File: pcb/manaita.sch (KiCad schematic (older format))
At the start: 110 parts, among them J1 SCK, J2 RST, J3 MOSI, J4 MISO, J5 VCC, J6 GND, U1 ATmega32U4-AU, Y1 Crystal_GND24_Small

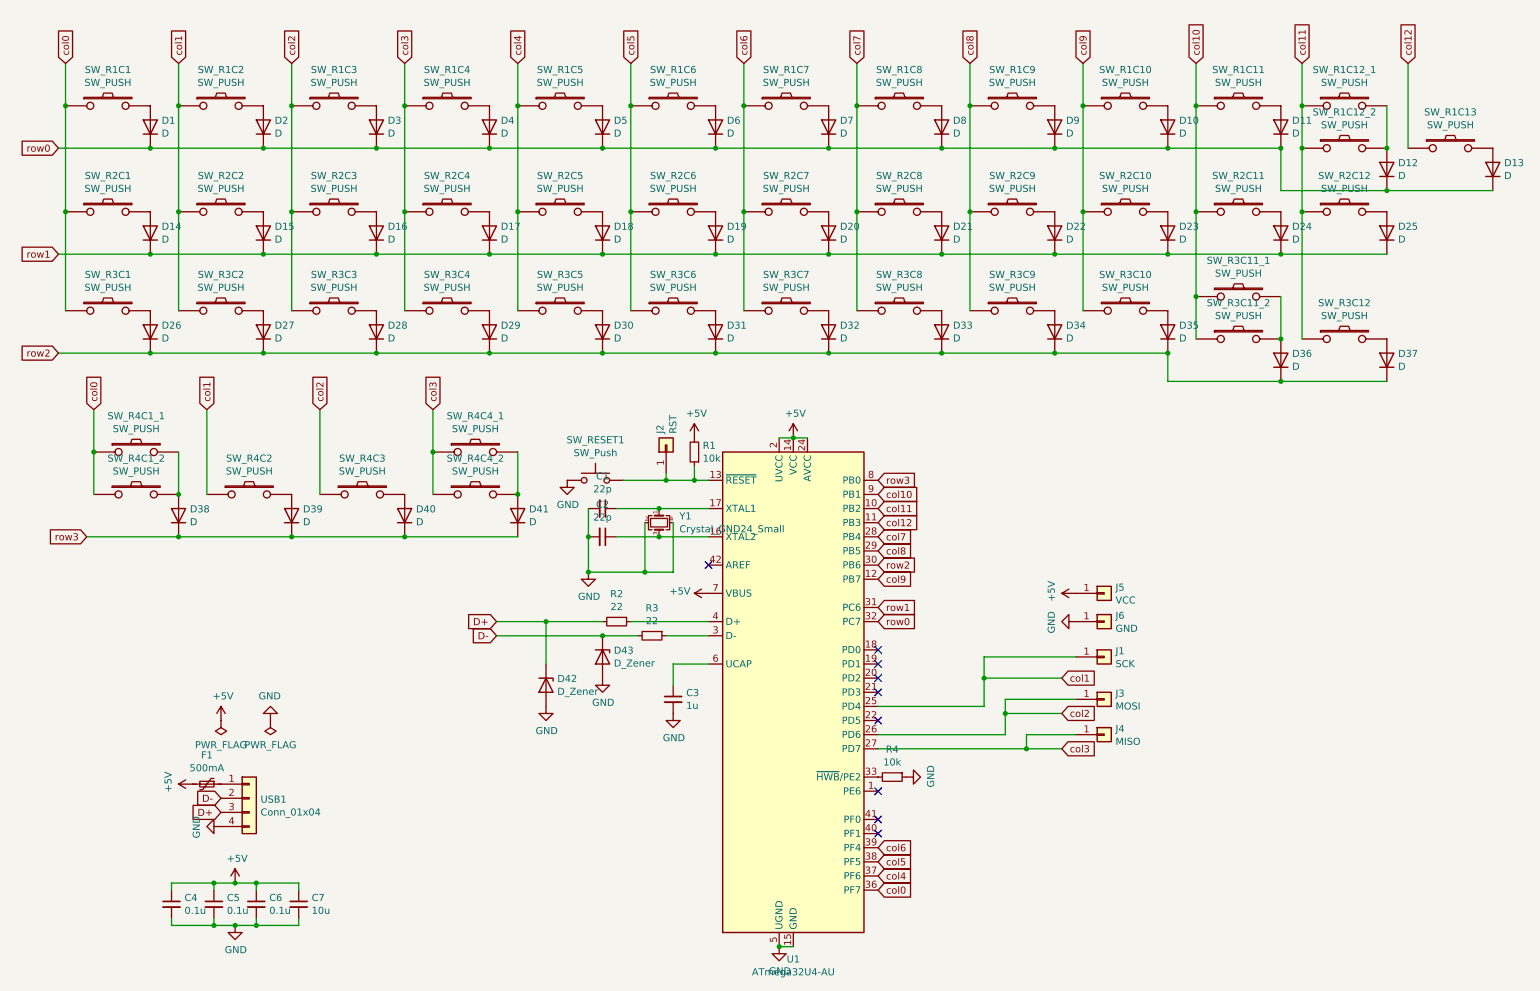
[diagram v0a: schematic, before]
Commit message: create pcb done
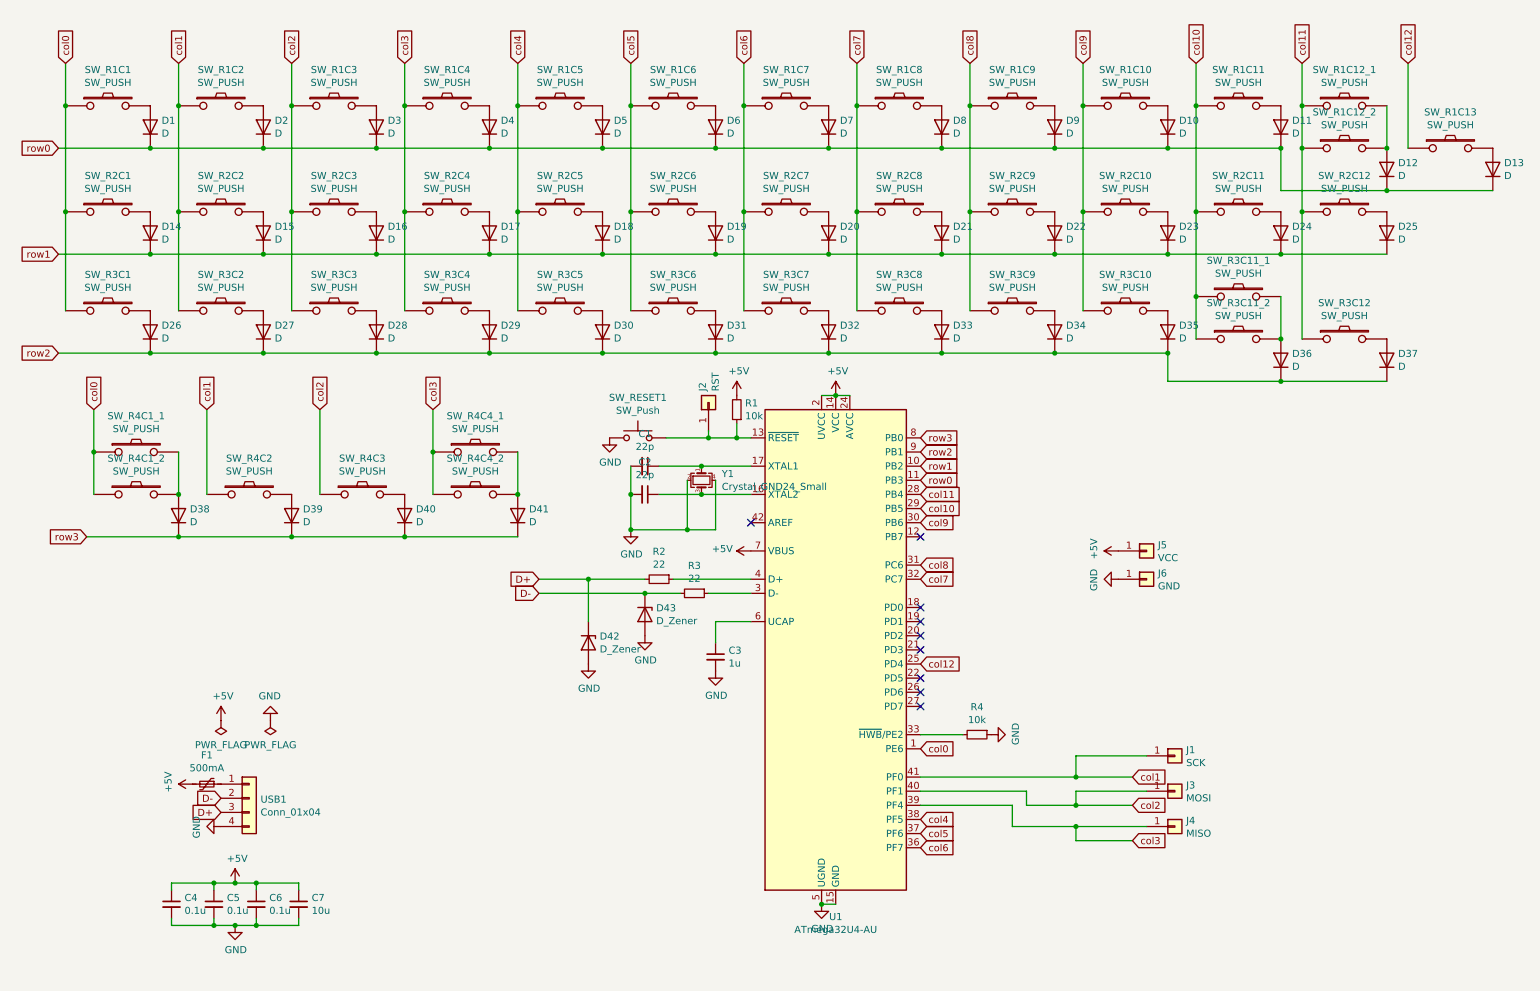
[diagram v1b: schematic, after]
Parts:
- D1, D10, D11, D12, D13, D14, D15, D16, D17, D18, D19, D2, D20, D21, D22, D23, D24, D25, D26, D27, D28, D29, D3, D30, D31, D32, D33, D34, D35, D36, D37, D38, D39, D4, D40, D41, D5, D6, D7, D8, D9: footprint swanmatch:D3_SMD_v2 -> mikamo3:D3_SMD_1side
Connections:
- net col0: now also U1.1 (PE6); no longer U1.36 (PF7)
- net col1: now also U1.41 (PF0); no longer U1.25 (PD4)
- net col10: now also U1.29 (PB5); no longer U1.9 (PB1)
- net col11: now also U1.28 (PB4); no longer U1.10 (PB2)
- net col12: now also U1.25 (PD4); no longer U1.11 (PB3)
- net col2: now also U1.40 (PF1); no longer U1.26 (PD6)
- net col3: now also U1.39 (PF4); no longer U1.27 (PD7)
- net col4: now also U1.38 (PF5); no longer U1.37 (PF6)
- net col5: now also U1.37 (PF6); no longer U1.38 (PF5)
- net col6: now also U1.36 (PF7); no longer U1.39 (PF4)
- net col7: now also U1.32 (PC7); no longer U1.28 (PB4)
- net col8: now also U1.31 (PC6); no longer U1.29 (PB5)
- net col9: now also U1.30 (PB6); no longer U1.12 (PB7)
- net row0: now also U1.11 (PB3); no longer U1.32 (PC7)
- net row1: now also U1.10 (PB2); no longer U1.31 (PC6)
- net row2: now also U1.9 (PB1); no longer U1.30 (PB6)
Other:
- moved on the sheet: C1, C2, C3, D42, D43, J1, J2, J3, J4, J5, J6, R1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

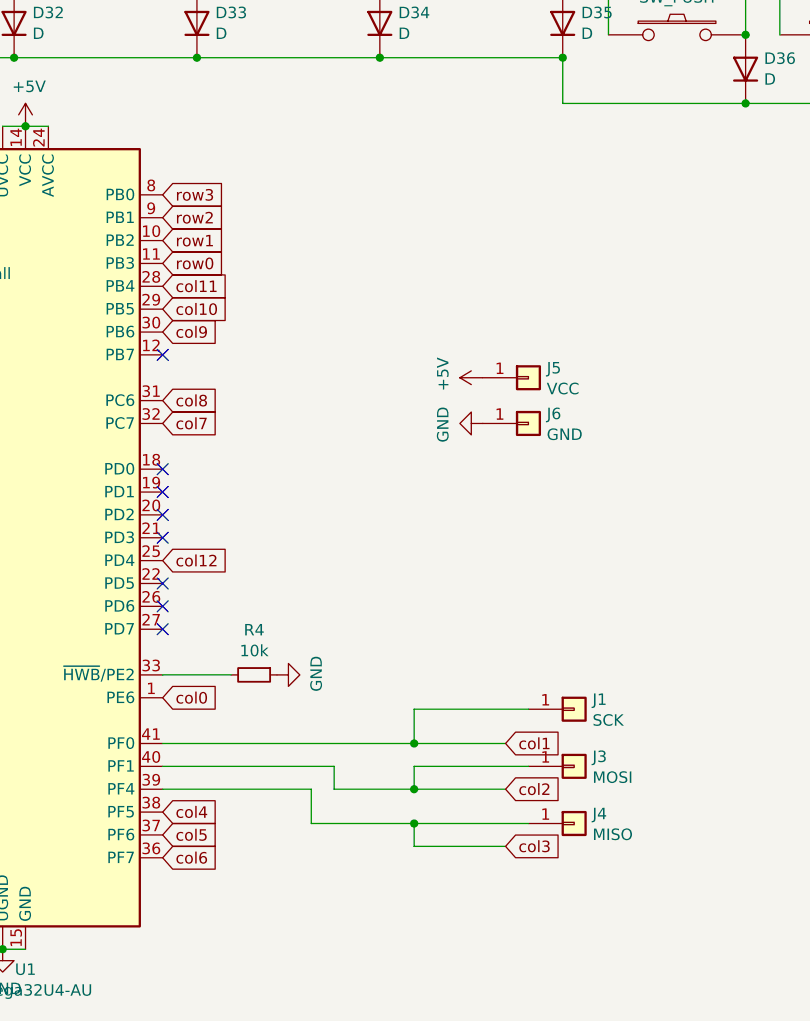
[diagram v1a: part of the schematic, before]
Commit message: :sparkles: (pcb) fix chore
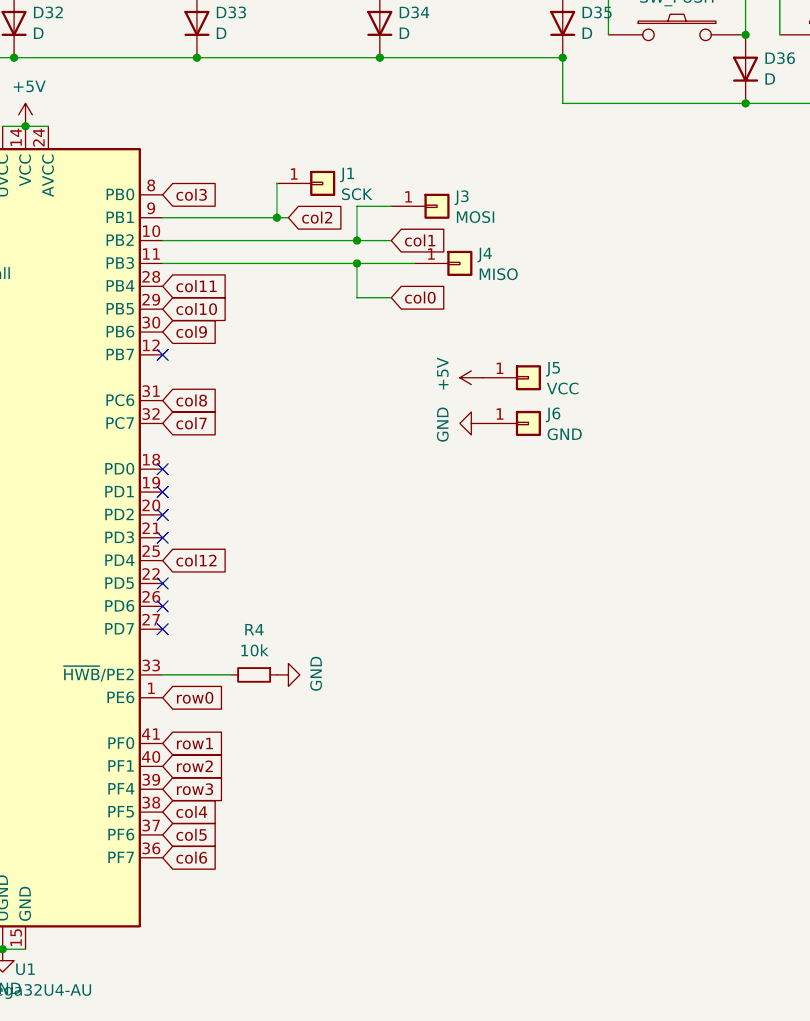
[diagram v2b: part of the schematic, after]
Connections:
- net col0: now also J4.1 (Pin_1), U1.11 (PB3); no longer U1.1 (PE6)
- net col1: now also J3.1 (Pin_1), U1.10 (PB2); no longer J1.1 (Pin_1), U1.41 (PF0)
- net col2: now also J1.1 (Pin_1), U1.9 (PB1); no longer J3.1 (Pin_1), U1.40 (PF1)
- net col3: now also U1.8 (PB0); no longer J4.1 (Pin_1), U1.39 (PF4)
- net row0: now also U1.1 (PE6); no longer U1.11 (PB3)
- net row1: now also U1.41 (PF0); no longer U1.10 (PB2)
- net row2: now also U1.40 (PF1); no longer U1.9 (PB1)
- net row3: now also U1.39 (PF4); no longer U1.8 (PB0)
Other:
- moved on the sheet: J1, J3, J4
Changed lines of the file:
@@
 	4800 3600 4800 3800
 Connection ~ 4800 3800
-Text GLabel 6850 3700 2    50   Input ~ 0
+Text GLabel 6850 5600 2    50   Input ~ 0
 row0
-Text GLabel 6850 3500 2    50   Input ~ 0
+Text GLabel 6850 5900 2    50   Input ~ 0
 row2
-Text GLabel 6850 3600 2    50   Input ~ 0
+Text GLabel 6850 5800 2    50   Input ~ 0
 row1
+Text GLabel 6850 6000 2    50   Input ~ 0
+row3
+Text GLabel 7850 3850 2    50   Input ~ 0
+col0
+Text GLabel 7850 3600 2    50   Input ~ 0
+col1
+Text GLabel 7400 3500 2    50   Input ~ 0
+col2
 Text GLabel 6850 3400 2    50   Input ~ 0
-row3
-Text GLabel 6850 5600 2    50   Input ~ 0
-col0
-Text GLabel 8350 5800 2    50   Input ~ 0
-col1
-Text GLabel 8350 6000 2    50   Input ~ 0
-col2
-Text GLabel 8350 6250 2    50   Input ~ 0
 col3
 Text GLabel 6850 6100 2    50   Input ~ 0
@@
 L Connector_Generic:Conn_01x01 J4
 U 1 1 5FB79428
-P 8650 6150
-F 0 "J4" H 8730 6192 50  0000 L CNN
-F 1 "MISO" H 8730 6101 50  0000 L CNN
-F 2 "swanmatch:1pin_conn" H 8650 6150 50  0001 C CNN
-F 3 "~" H 8650 6150 50  0001 C CNN
-	1    8650 6150
+P 8150 3700
+F 0 "J4" H 8230 3742 50  0000 L CNN
+F 1 "MISO" H 8230 3651 50  0000 L CNN
+F 2 "swanmatch:1pin_conn" H 8150 3700 50  0001 C CNN
+F 3 "~" H 8150 3700 50  0001 C CNN
+	1    8150 3700
 	1    0    0    -1
 $EndComp
@@
 L Connector_Generic:Conn_01x01 J3
 U 1 1 5FB79976
-P 8650 5900
-F 0 "J3" H 8730 5942 50  0000 L CNN
-F 1 "MOSI" H 8730 5851 50  0000 L CNN
-F 2 "swanmatch:1pin_conn" H 8650 5900 50  0001 C CNN
-F 3 "~" H 8650 5900 50  0001 C CNN
-	1    8650 5900
+P 8050 3450
+F 0 "J3" H 8130 3492 50  0000 L CNN
+F 1 "MOSI" H 8130 3401 50  0000 L CNN
+F 2 "swanmatch:1pin_conn" H 8050 3450 50  0001 C CNN
+F 3 "~" H 8050 3450 50  0001 C CNN
+	1    8050 3450
 	1    0    0    -1
 $EndComp
@@
 L Connector_Generic:Conn_01x01 J1
 U 1 1 5FB79F9C
-P 8650 5650
-F 0 "J1" H 8730 5692 50  0000 L CNN
-F 1 "SCK" H 8730 5601 50  0000 L CNN
-F 2 "swanmatch:1pin_conn" H 8650 5650 50  0001 C CNN
-F 3 "~" H 8650 5650 50  0001 C CNN
-	1    8650 5650
+P 7550 3350
+F 0 "J1" H 7630 3392 50  0000 L CNN
+F 1 "SCK" H 7630 3301 50  0000 L CNN
+F 2 "swanmatch:1pin_conn" H 7550 3350 50  0001 C CNN
+F 3 "~" H 7550 3350 50  0001 C CNN
+	1    7550 3350
 	1    0    0    -1
 $EndComp
@@
 	0    -1   -1   0
 $EndComp
-Wire Wire Line
-	7600 6000 7950 6000
-Wire Wire Line
-	7950 6000 8350 6000
-Wire Wire Line
-	8450 5900 7950 5900
-Wire Wire Line
-	6850 5800 7950 5800
-Wire Wire Line
-	7950 5800 8350 5800
-Wire Wire Line
-	8450 5650 7950 5650
-Wire Wire Line
-	7950 5650 7950 5800
-Connection ~ 7950 5800
 $Comp
 L power:GND #PWR06
@@
 Wire Wire Line
 	4500 4400 4900 4400
-Connection ~ 7950 6000
-Wire Wire Line
-	7950 5900 7950 6000
-Wire Wire Line
-	8350 6250 7950 6250
-Wire Wire Line
-	7950 6250 7950 6150
-Connection ~ 7950 6150
-Wire Wire Line
-	7950 6150 8450 6150
 Wire Wire Line
 	6850 5500 7150 5500
 Text GLabel 4150 4500 0    50   Input ~ 0
 D-
-Wire Wire Line
-	6850 5900 7600 5900
-Wire Wire Line
-	7600 5900 7600 6000
-Wire Wire Line
-	6850 6000 7500 6000
-Wire Wire Line
-	7500 6000 7500 6150
-Wire Wire Line
-	7500 6150 7950 6150
 $Comp
 L MCU_Microchip_ATmega:ATmega32U4-AU U1
@@
 NoConn ~ 6850 5300
 NoConn ~ 6850 4100
+Wire Wire Line
+	6850 3500 7350 3500
+Wire Wire Line
+	7350 3500 7350 3350
+Wire Wire Line
+	7350 3500 7400 3500
+Connection ~ 7350 3500
+Wire Wire Line
+	6850 3600 7700 3600
+Wire Wire Line
+	7850 3450 7700 3450
+Wire Wire Line
+	7700 3450 7700 3600
+Connection ~ 7700 3600
+Wire Wire Line
+	7700 3600 7850 3600
+Wire Wire Line
+	6850 3700 7700 3700
+Wire Wire Line
+	7700 3700 7700 3850
+Wire Wire Line
+	7700 3850 7850 3850
+Connection ~ 7700 3700
+Wire Wire Line
+	7700 3700 7950 3700
 $EndSCHEMATC
